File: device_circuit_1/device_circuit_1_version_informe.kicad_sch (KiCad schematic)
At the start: 18 parts, among them J1 5 V, J2 Conn_01x15_Male, J3 Conn_01x15_Male, J4 SENSOR DE PROXIMIDAD MAGNÉTICO, J9 Screw_Terminal_01x03, U1 OP77

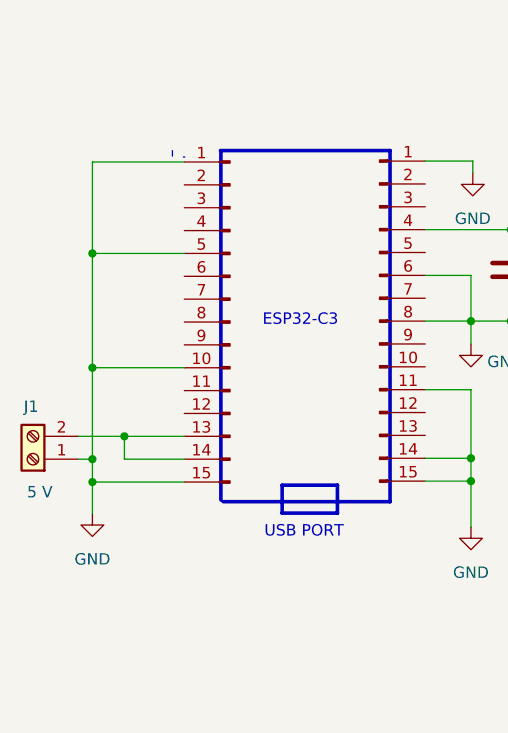
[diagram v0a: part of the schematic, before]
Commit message: actualizado repo
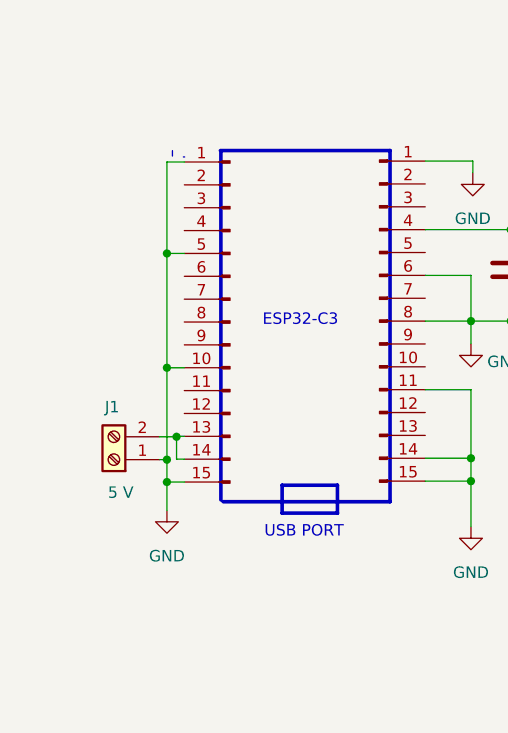
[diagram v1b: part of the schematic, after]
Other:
- moved on the sheet: J1
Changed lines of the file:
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@@
 (kicad_sch (version 20211123) (generator eeschema)
   (paper "A4")
+  (junction (at 52.8828 92.8116) (diameter 0) (color 0 0 0 0)
+  )
   (junction (at 116.4844 67.3608) (diameter 0) (color 0 0 0 0)
   )
@@
   (junction (at 167.2844 58.4708) (diameter 0) (color 0 0 0 0)
   )
+  (junction (at 52.8828 69.9008) (diameter 0) (color 0 0 0 0)
+  )
+  (junction (at 52.8828 95.3008) (diameter 0) (color 0 0 0 0)
+  )
   (junction (at 91.0844 77.4192) (diameter 0) (color 0 0 0 0)
   )
-  (junction (at 44.6024 69.9008) (diameter 0) (color 0 0 0 0)
-  )
   (junction (at 86.6648 92.6592) (diameter 0) (color 0 0 0 0)
   )
   (junction (at 91.0844 67.2592) (diameter 0) (color 0 0 0 0)
   )
-  (junction (at 44.6024 95.3008) (diameter 0) (color 0 0 0 0)
-  )
   (junction (at 163.4744 77.5208) (diameter 0) (color 0 0 0 0)
   )
@@
   (junction (at 144.4244 64.8208) (diameter 0) (color 0 0 0 0)
   )
-  (junction (at 44.6024 82.6008) (diameter 0) (color 0 0 0 0)
-  )
-  (junction (at 48.1584 90.2208) (diameter 0) (color 0 0 0 0)
+  (junction (at 52.8828 82.6008) (diameter 0) (color 0 0 0 0)
   )
   (junction (at 86.6648 77.4192) (diameter 0) (color 0 0 0 0)
@@
   (junction (at 172.3644 87.6808) (diameter 0) (color 0 0 0 0)
   )
-  (junction (at 44.6024 92.7608) (diameter 0) (color 0 0 0 0)
+  (junction (at 53.9496 90.2716) (diameter 0) (color 0 0 0 0)
   )
   (junction (at 86.6648 95.1992) (diameter 0) (color 0 0 0 0)
@@
     (stroke (width 0) (type default) (color 0 0 0 0))
   )
+  (wire (pts (xy 52.07 92.8116) (xy 52.8828 92.8116))
+    (stroke (width 0) (type default) (color 0 0 0 0))
+  )
   (wire (pts (xy 86.868 59.6392) (xy 86.868 60.96))
     (stroke (width 0) (type default) (color 0 0 0 0))
@@
   )
   (wire (pts (xy 163.4744 47.0408) (xy 172.3644 47.0408))
+    (stroke (width 0) (type default) (color 0 0 0 0))
+  )
+  (wire (pts (xy 52.8828 69.9008) (xy 52.8828 82.6008))
     (stroke (width 0) (type default) (color 0 0 0 0))
   )
@@
     (stroke (width 0) (type default) (color 0 0 0 0))
   )
-  (wire (pts (xy 54.8132 95.3008) (xy 44.6024 95.3008))
+  (wire (pts (xy 54.8132 95.3008) (xy 52.8828 95.3008))
     (stroke (width 0) (type default) (color 0 0 0 0))
   )
@@
     (stroke (width 0) (type default) (color 0 0 0 0))
   )
-  (wire (pts (xy 44.6024 82.6008) (xy 54.8132 82.6008))
+  (wire (pts (xy 54.8132 92.7608) (xy 53.9496 92.7608))
     (stroke (width 0) (type default) (color 0 0 0 0))
   )
@@
     (stroke (width 0) (type default) (color 0 0 0 0))
   )
+  (wire (pts (xy 52.8828 82.6008) (xy 54.8132 82.6008))
+    (stroke (width 0) (type default) (color 0 0 0 0))
+  )
   (wire (pts (xy 172.3644 86.4108) (xy 172.3644 87.6808))
+    (stroke (width 0) (type default) (color 0 0 0 0))
+  )
+  (wire (pts (xy 52.8828 69.9008) (xy 54.8132 69.9008))
     (stroke (width 0) (type default) (color 0 0 0 0))
   )
@@
     (stroke (width 0) (type default) (color 0 0 0 0))
   )
-  (wire (pts (xy 48.1584 92.7608) (xy 48.1584 90.2208))
-    (stroke (width 0) (type default) (color 0 0 0 0))
-  )
   (wire (pts (xy 158.3944 69.9008) (xy 154.5844 69.9008))
     (stroke (width 0) (type default) (color 0 0 0 0))
@@
     (stroke (width 0.4) (type solid) (color 132 0 0 1))
   )
+  (wire (pts (xy 52.8828 59.7408) (xy 52.8828 69.9008))
+    (stroke (width 0) (type default) (color 0 0 0 0))
+  )
   (wire (pts (xy 124.1044 97.8408) (xy 116.4844 97.8408))
     (stroke (width 0) (type default) (color 0 0 0 0))
   )
-  (wire (pts (xy 44.6024 69.9008) (xy 44.6024 59.7408))
-    (stroke (width 0) (type default) (color 0 0 0 0))
-  )
   (wire (pts (xy 136.8044 59.7408) (xy 136.8044 47.0408))
     (stroke (width 0) (type default) (color 0 0 0 0))
@@
     (stroke (width 0) (type default) (color 0 0 0 0))
   )
+  (wire (pts (xy 52.8828 82.6008) (xy 52.8828 92.8116))
+    (stroke (width 0) (type default) (color 0 0 0 0))
+  )
   (wire (pts (xy 81.5848 67.2592) (xy 91.0844 67.2592))
     (stroke (width 0) (type default) (color 0 0 0 0))
@@
     (stroke (width 0) (type default) (color 0 0 0 0))
   )
-  (wire (pts (xy 54.8132 90.2208) (xy 48.1584 90.2208))
-    (stroke (width 0) (type default) (color 0 0 0 0))
-  )
   (wire (pts (xy 120.2944 74.9808) (xy 131.7244 74.9808))
     (stroke (width 0) (type default) (color 0 0 0 0))
@@
     (stroke (width 0) (type default) (color 0 0 0 0))
   )
+  (wire (pts (xy 53.9496 90.2716) (xy 53.9496 92.7608))
+    (stroke (width 0) (type default) (color 0 0 0 0))
+  )
   (wire (pts (xy 199.0344 52.1208) (xy 195.2244 52.1208))
     (stroke (width 0) (type default) (color 0 0 0 0))
@@
     (stroke (width 0) (type default) (color 0 0 0 0))
   )
-  (wire (pts (xy 44.6024 69.9008) (xy 54.8132 69.9008))
+  (wire (pts (xy 52.07 90.2716) (xy 53.9496 90.2716))
     (stroke (width 0) (type default) (color 0 0 0 0))
   )
@@
     (stroke (width 0) (type default) (color 0 0 0 0))
   )
-  (wire (pts (xy 54.8132 92.7608) (xy 48.1584 92.7608))
+  (wire (pts (xy 53.9496 90.2208) (xy 53.9496 90.2716))
     (stroke (width 0) (type default) (color 0 0 0 0))
   )
@@
     (stroke (width 0) (type default) (color 0 0 0 0))
   )
+  (wire (pts (xy 52.8828 95.3008) (xy 52.8828 98.4504))
+    (stroke (width 0) (type default) (color 0 0 0 0))
+  )
   (wire (pts (xy 144.4244 64.8208) (xy 146.9644 64.8208))
     (stroke (width 0) (type default) (color 0 0 0 0))
   )
   (wire (pts (xy 120.2944 74.9808) (xy 120.2944 86.4108))
-    (stroke (width 0) (type default) (color 0 0 0 0))
-  )
-  (wire (pts (xy 43.0784 92.7608) (xy 44.6024 92.7608))
     (stroke (width 0) (type default) (color 0 0 0 0))
   )
@@
     (stroke (width 0) (type default) (color 0 0 0 0))
   )
-  (wire (pts (xy 44.6024 59.7408) (xy 54.8132 59.7408))
-    (stroke (width 0) (type default) (color 0 0 0 0))
-  )
   (wire (pts (xy 91.0844 67.2592) (xy 102.2604 67.2592))
     (stroke (width 0) (type default) (color 0 0 0 0))
@@
     (stroke (width 0) (type default) (color 0 0 0 0))
   )
-  (wire (pts (xy 44.6024 95.3008) (xy 44.6024 98.806))
+  (wire (pts (xy 52.8828 59.7408) (xy 54.8132 59.7408))
     (stroke (width 0) (type default) (color 0 0 0 0))
   )
@@
     (stroke (width 0) (type default) (color 0 0 0 0))
   )
-  (wire (pts (xy 44.6024 82.6008) (xy 44.6024 69.9008))
+  (wire (pts (xy 52.8828 92.8116) (xy 52.8828 95.3008))
     (stroke (width 0) (type default) (color 0 0 0 0))
   )
@@
     (stroke (width 0) (type default) (color 0 0 0 0))
   )
+  (wire (pts (xy 53.9496 90.2208) (xy 54.8132 90.2208))
+    (stroke (width 0) (type default) (color 0 0 0 0))
+  )
   (polyline (pts (xy 53.4924 58.4708) (xy 53.4924 59.0804))
     (stroke (width 0) (type default) (color 0 0 0 0))
   )
-  (wire (pts (xy 44.6024 92.7608) (xy 44.6024 95.3008))
-    (stroke (width 0) (type default) (color 0 0 0 0))
-  )
   (wire (pts (xy 114.3 67.3608) (xy 116.4844 67.3608))
-    (stroke (width 0) (type default) (color 0 0 0 0))
-  )
-  (wire (pts (xy 48.1584 90.2208) (xy 43.0784 90.2208))
-    (stroke (width 0) (type default) (color 0 0 0 0))
-  )
-  (wire (pts (xy 44.6024 82.6008) (xy 44.6024 92.7608))
     (stroke (width 0) (type default) (color 0 0 0 0))
   )
@@
     (pin "1")
   )
-  (symbol (lib_id "power:GND") (at 44.6024 98.806 0) (unit 1)
+  (symbol (lib_id "power:GND") (at 52.8828 98.4504 0) (unit 1)
     (in_bom yes) (on_board yes) (fields_autoplaced)
-    (property "Reference" "#PWR01" (id 0) (at 44.6024 105.156 0)
-      (effects (font (size 1.27 1.27)) hide)
-    )
-    (property "Value" "GND" (id 1) (at 44.6024 103.886 0))
-    (property "Footprint" "" (id 2) (at 44.6024 98.806 0)
-      (effects (font (size 1.27 1.27)) hide)
-    )
-    (property "Datasheet" "" (id 3) (at 44.6024 98.806 0)
+    (property "Reference" "#PWR01" (id 0) (at 52.8828 104.8004 0)
+      (effects (font (size 1.27 1.27)) hide)
+    )
+    (property "Value" "GND" (id 1) (at 52.8828 103.5304 0))
+    (property "Footprint" "" (id 2) (at 52.8828 98.4504 0)
+      (effects (font (size 1.27 1.27)) hide)
+    )
+    (property "Datasheet" "" (id 3) (at 52.8828 98.4504 0)
       (effects (font (size 1.27 1.27)) hide)
     )
@@
     (pin "1")
   )
-  (symbol (lib_id "Connector:Screw_Terminal_01x02") (at 37.9984 92.7608 180) (unit 1)
-    (in_bom yes) (on_board yes)
-    (property "Reference" "J1" (id 0) (at 37.7952 86.9188 0))
-    (property "Value" "5 V" (id 1) (at 38.7604 96.4184 0))
-    (property "Footprint" "Connector_Phoenix_MC_HighVoltage:PhoenixContact_MCV_1,5_2-G-5.08_1x02_P5.08mm_Vertical" (id 2) (at 37.9984 92.7608 0)
-      (effects (font (size 1.27 1.27)) hide)
-    )
-    (property "Datasheet" "~" (id 3) (at 37.9984 92.7608 0)
-      (effects (font (size 1.27 1.27)) hide)
-    )
+  (symbol (lib_id "Connector:Screw_Terminal_01x02") (at 46.99 92.8116 180) (unit 1)
+    (in_bom yes) (on_board yes)
+    (property "Reference" "J1" (id 0) (at 46.7868 86.9696 0))
+    (property "Value" "5 V" (id 1) (at 47.752 96.4692 0))
+    (property "Footprint" "Connector_Phoenix_MC_HighVoltage:PhoenixContact_MCV_1,5_2-G-5.08_1x02_P5.08mm_Vertical" (id 2) (at 46.99 92.8116 0)
+      (effects (font (size 1.27 1.27)) hide)
+    )
+    (property "Datasheet" "~" (id 3) (at 46.99 92.8116 0)
+      (effects (font (size 1.27 1.27)) hide)
+    )
